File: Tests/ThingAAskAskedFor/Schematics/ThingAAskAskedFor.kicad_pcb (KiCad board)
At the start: 2 copper layers, 41.5 x 54 mm, 10 parts, among them U1 Pico, U12 SW3, U15 SW_Push, U16 SW_Push, U18 100nF, U20 SK6812, U4 Conn_02x03_Odd_Even, U6 100nF, U7 Buzzer, U9 SK6812

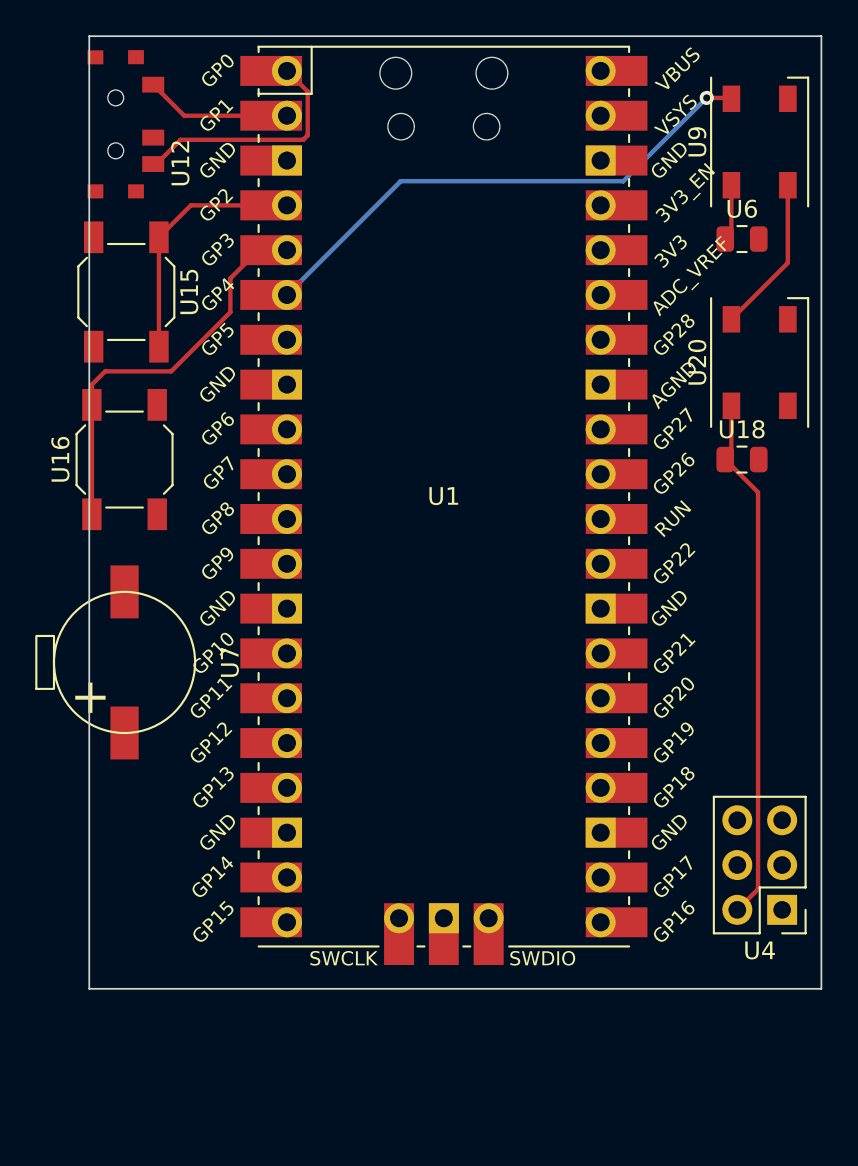
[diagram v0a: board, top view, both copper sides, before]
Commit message: Updating for picoducky
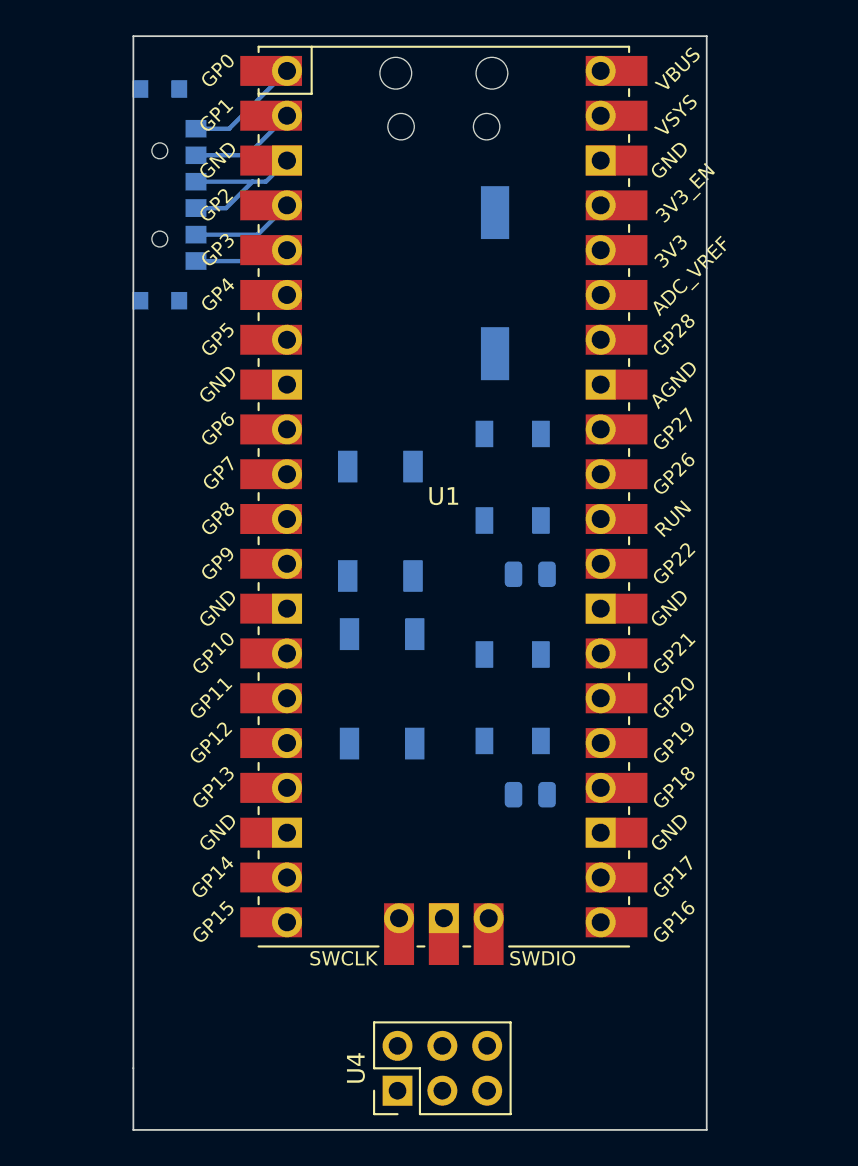
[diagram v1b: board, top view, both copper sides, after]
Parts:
- removed U12: SW3, BreadBoardPwr:SK-3296S_switch
- added J1: Conn_01x06, ThingAAskAskedFor:MK-14C01-G2 SP4T Switch, B.Cu at (131.5, 68.0)
- U15, U16, U18, U20, U6, U7, U9: moved to B.Cu
- moved U7 30.1 mm to (150.5, 77.0)
- moved U4 24.1 mm to (145.0, 118.8), turned to 90 degrees
- moved U20 23.6 mm to (151.5, 96.5)
- moved U9 23.6 mm to (151.5, 84.0)
- moved U18 22.5 mm to (152.5, 102.0), turned to 180 degrees
- moved U6 22.5 mm to (152.5, 89.5), turned to 180 degrees
- moved U16 19.5 mm to (144.1, 96.0)
- moved U15 19.4 mm to (144.0, 86.5)
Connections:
- U1 pad 13: unconnected-(U1-GND)_1 -> VSS
- U1 pad 18: unconnected-(U1-GND)_2 -> VSS
- U1 pad 23: unconnected-(U1-GND)_3 -> VSS
- U1 pad 28: unconnected-(U1-GND)_4 -> VSS
- U1 pad 3: unconnected-(U1-GND)_5 -> VSS
- U1 pad 33: unconnected-(U1-AGND) -> VSS
- U1 pad 38: unconnected-(U1-GND)_6 -> VSS
- U1 pad 4: Button1 -> 3
- U1 pad 42: unconnected-(U1-GND)_7 -> VSS
- U1 pad 5: Button2 -> 4
- U1 pad 6: /SK6812 -> Button1
- U1 pad 7: Buzzer -> Button2
- U1 pad 8: unconnected-(U1-GND) -> VSS
- U4 pad 6: Cout -> unconnected-(U4-Pin_6)
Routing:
- net VCC: track 33.2 -> 0.00 mm
- net /SK6812: track 29.8 -> 0.00 mm, vias 1 -> 0
- net Button2: track 22.7 -> 0.00 mm
- net Button1: track 14.2 -> 0.00 mm
- net VSS: track 0.00 -> 9.48 mm
- net Net-(U20-DIN): track 8.93 -> 0.00 mm
- net 1: track 13.6 -> 6.52 mm
- net 3: track 0.00 -> 5.85 mm
- net 4: track 0.00 -> 5.42 mm
- net 2: track 8.31 -> 6.09 mm
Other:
- board size 41.5 x 54 mm -> 32.5 x 62 mm
